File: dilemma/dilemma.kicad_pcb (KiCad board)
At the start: 2 copper layers, 134 x 95.1 mm, 82 parts, among them J1 S3B-PH-SM4-TB(LF)(SN), J2 Serial, J3 BATTERY_CONN_DEANS, J5 S3B-PH-SM4-TB(LF)(SN), SW1 SW_Push, SW10 SW_Push, SW11 SW_Push, SW12 SW_Push, SW13 SW_Push, SW14 SW_Push, SW15 SW_Push, SW16 SW_Push, SW17 locked, SW2 SW_Push, SW26 SW_SPST, SW3 SW_Push, SW37 SW_SPST, SW4 SW_Push, SW5 SW_Push, SW6 SW_Push, SW7 SW_Push, SW8 SW_Push, SW9 SW_Push, U2 eliteC

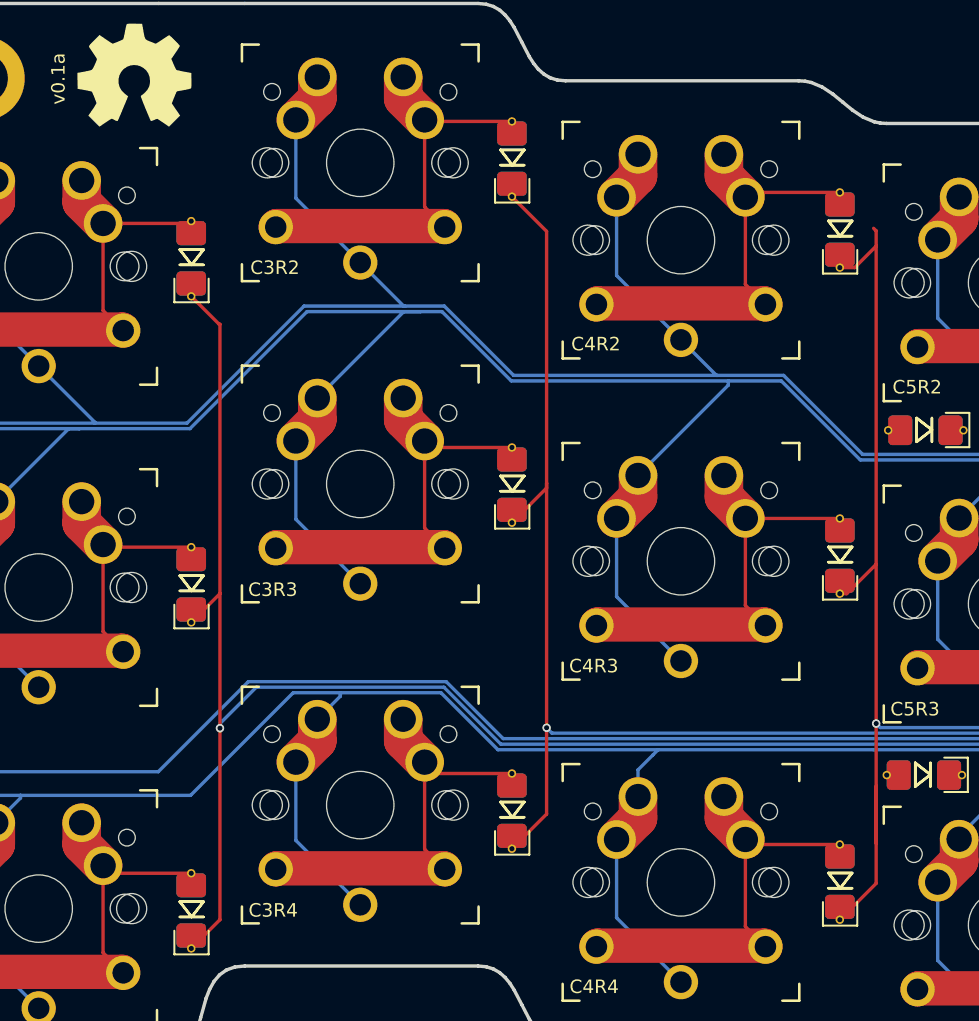
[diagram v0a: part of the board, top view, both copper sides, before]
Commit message: tenting puck
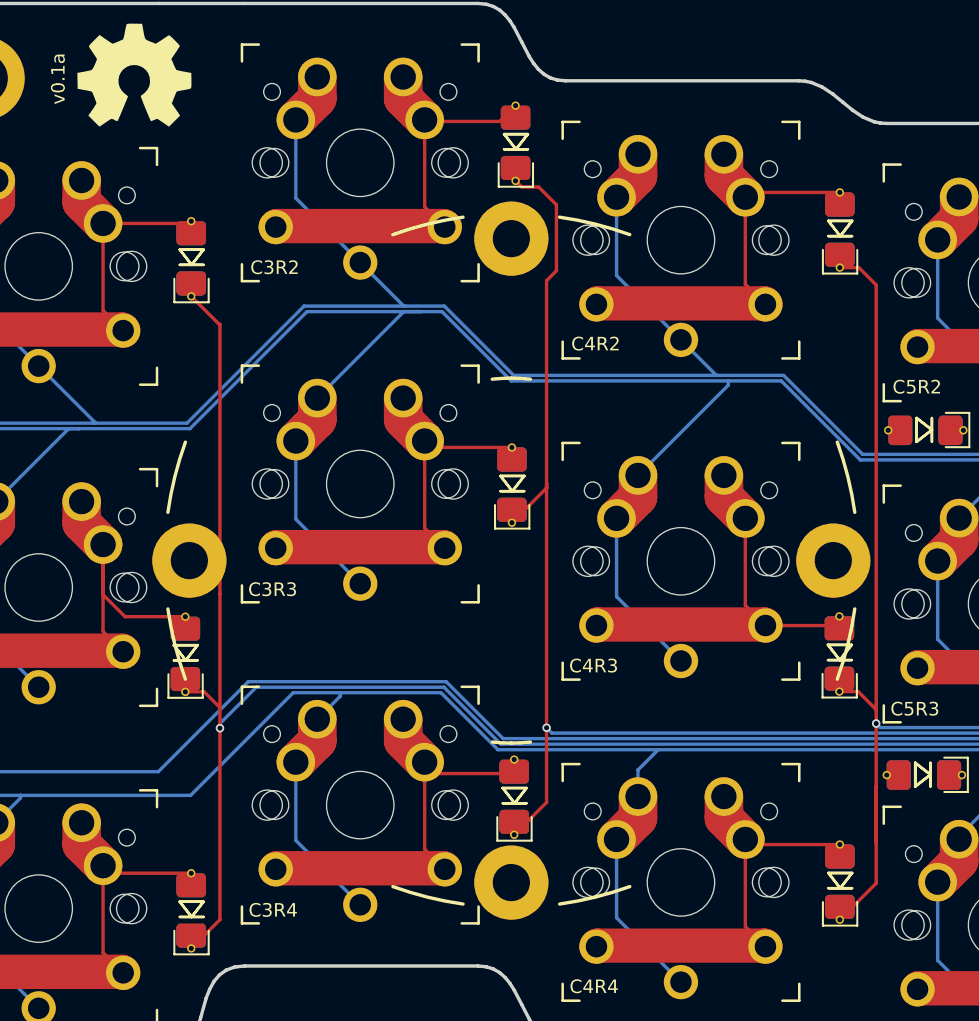
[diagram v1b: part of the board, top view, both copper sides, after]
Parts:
- added REF**: Tenting Puck, kbd:Tenting_Puck2, F.Cu at (162.4, 56.6)
- moved D19 5.79 mm to (181.8, 62.1)
- moved D9 4.13 mm to (143.1, 62.1)
- moved D13 0.96 mm to (162.6, 31.9)
- moved D15 0.84 mm to (162.6, 70.6)
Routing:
- net col4_l: track 84.6 -> 80.8 mm
- net Net-(D9-Pad2): track 25.2 -> 28.3 mm
- net col3_l: track 116.3 -> 117.6 mm
- net Net-(D19-Pad2): track 25.5 -> 24.5 mm
- net Net-(D13-Pad2): track 25.2 -> 25.8 mm
